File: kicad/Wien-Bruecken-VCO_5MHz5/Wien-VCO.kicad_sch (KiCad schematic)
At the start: 22 parts, among them J1 J113, U1 ${SIM.NAME}

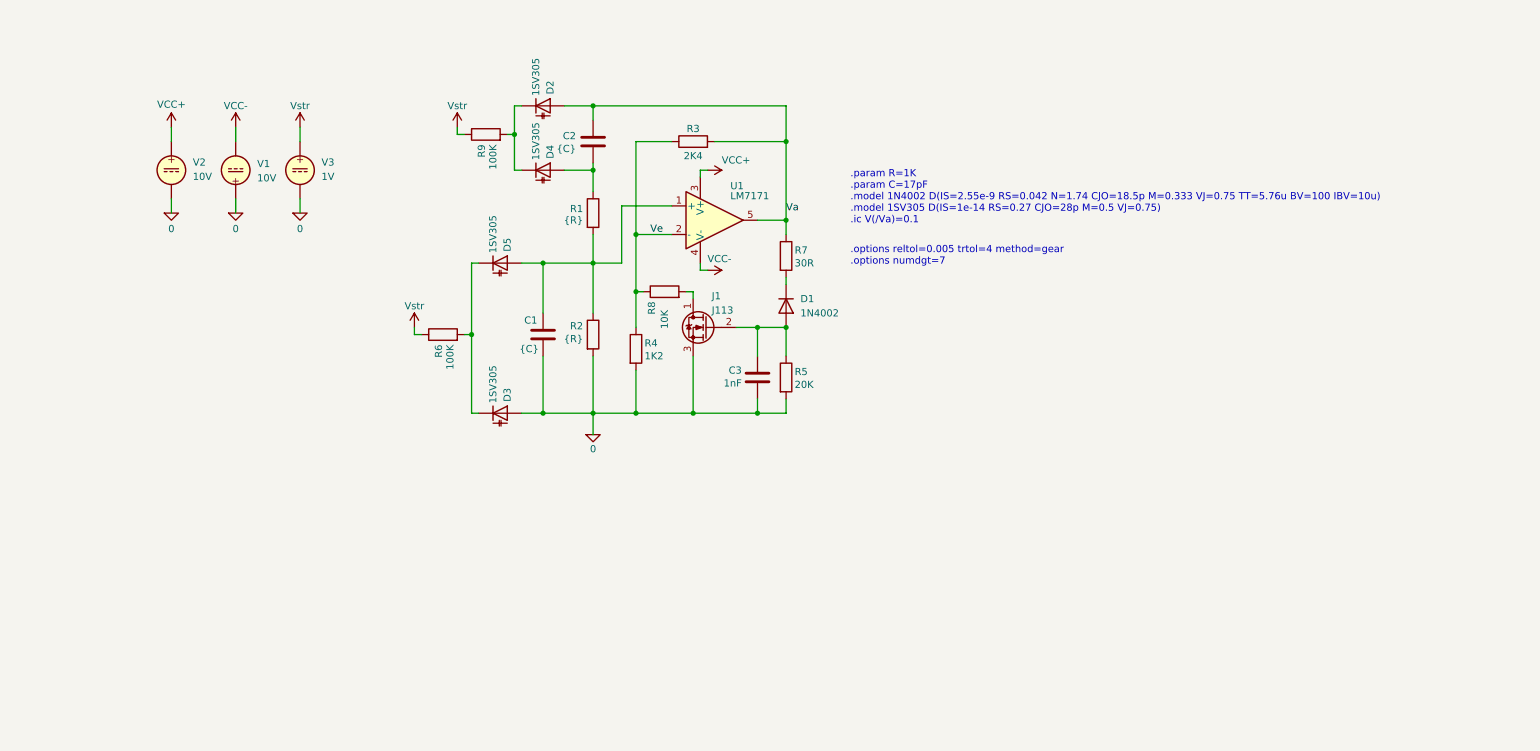
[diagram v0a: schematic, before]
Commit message: Kicad Schaltplan
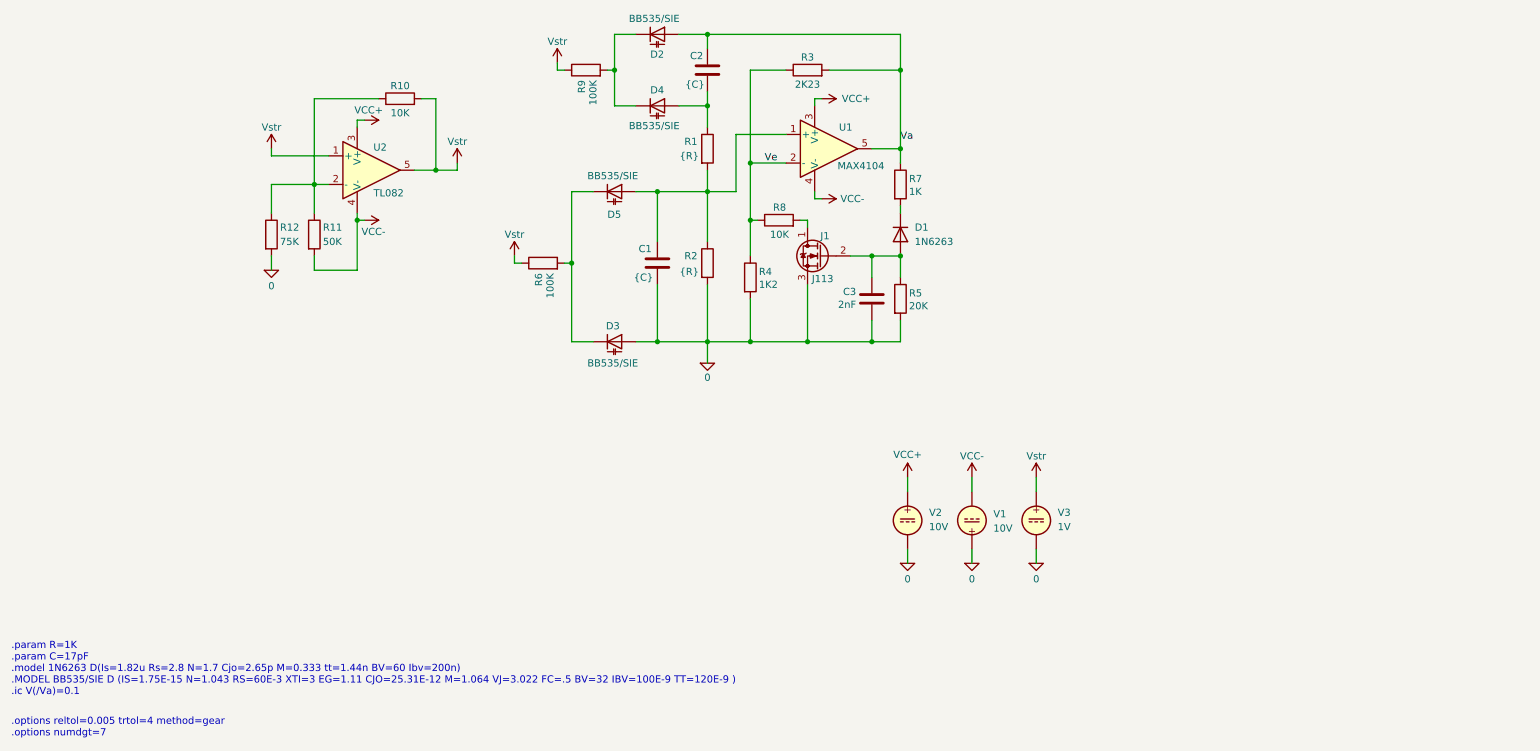
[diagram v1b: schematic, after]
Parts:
- added R10: 10K, Resistor_THT:R_Axial_DIN0207_L6.3mm_D2.5mm_P7.62mm_Horizontal, symbol Device:R
- added R11: 50K, Resistor_THT:R_Axial_DIN0207_L6.3mm_D2.5mm_P7.62mm_Horizontal, symbol Device:R
- added R12: 75K, Resistor_THT:R_Axial_DIN0207_L6.3mm_D2.5mm_P7.62mm_Horizontal, symbol Device:R
- added U2: ${SIM.NAME}, Library:TL082, symbol Simulation_SPICE:OPAMP
- C1, C2: footprint (none) -> Capacitor_THT:C_Rect_L10.0mm_W3.0mm_P7.50mm_MKS4
- C3: value 1nF -> 2nF; footprint (none) -> Capacitor_THT:C_Rect_L10.0mm_W3.0mm_P7.50mm_MKS4
- D1: value 1N4002 -> 1N6263
- D2, D3, D4, D5: value 1SV305 -> BB535/SIE; footprint (none) -> Diode_SMD:D_SOD-323F
- R1, R2, R4, R5, R6, R8, R9: footprint (none) -> Resistor_THT:R_Axial_DIN0207_L6.3mm_D2.5mm_P7.62mm_Horizontal
- R3: value 2K4 -> 2K23; footprint (none) -> Resistor_THT:R_Axial_DIN0207_L6.3mm_D2.5mm_P7.62mm_Horizontal
- R7: value 30R -> 1K; footprint (none) -> Resistor_THT:R_Axial_DIN0207_L6.3mm_D2.5mm_P7.62mm_Horizontal
- U1: footprint (none) -> Library:SOIC8-Adapter
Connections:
- net 0: now also R12.2
- net VCC+: now also U2.3 (V+)
- net VCC-: now also R11.2, U2.4 (V-)
- net Vstr: now also R10.2, U2.1 (+), U2.5
- new net: R10.1, R11.1, R12.1, U2.2 (-)
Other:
- note added: ".param R=1K .param C=17pF .model 1N6263 D(Is=1.82u Rs=2.8 N=1.7 Cjo=2.65p M=0.333 tt=1.44n BV=60 Ibv=200n) .MODEL BB535/SIE D (IS=1.75E-15 N=1.043 RS=60E-3 XTI=3 EG=1.11 CJO=25.31E-12 M=1.064 VJ=3.022 FC=.5 BV=32 IBV=100E-9 TT=120E-9 ) .ic V(/Va)=0.1"
- note removed: ".param R=1K .param C=17pF .model 1N4002 D(IS=2.55e-9 RS=0.042 N=1.74 CJO=18.5p M=0.333 VJ=0.75 TT=5.76u BV=100 IBV=10u) .model 1SV305 D(IS=1e-14 RS=0.27 CJO=28p M=0.5 VJ=0.75) .ic V(/Va)=0.1"
- moved on the sheet: C1, C2, C3, D1, D2, D3, D4, D5, J1, R1, R2, R3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
